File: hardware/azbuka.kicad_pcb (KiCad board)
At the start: 2 copper layers, 13 parts, among them IC1 ATTINY85-S, P1 USB_OTG, P2 CONN_01X06, Q1 MOSFET_P_CH, U1 AP111733, U2 TXS0102, U3 SJ1-3524NG

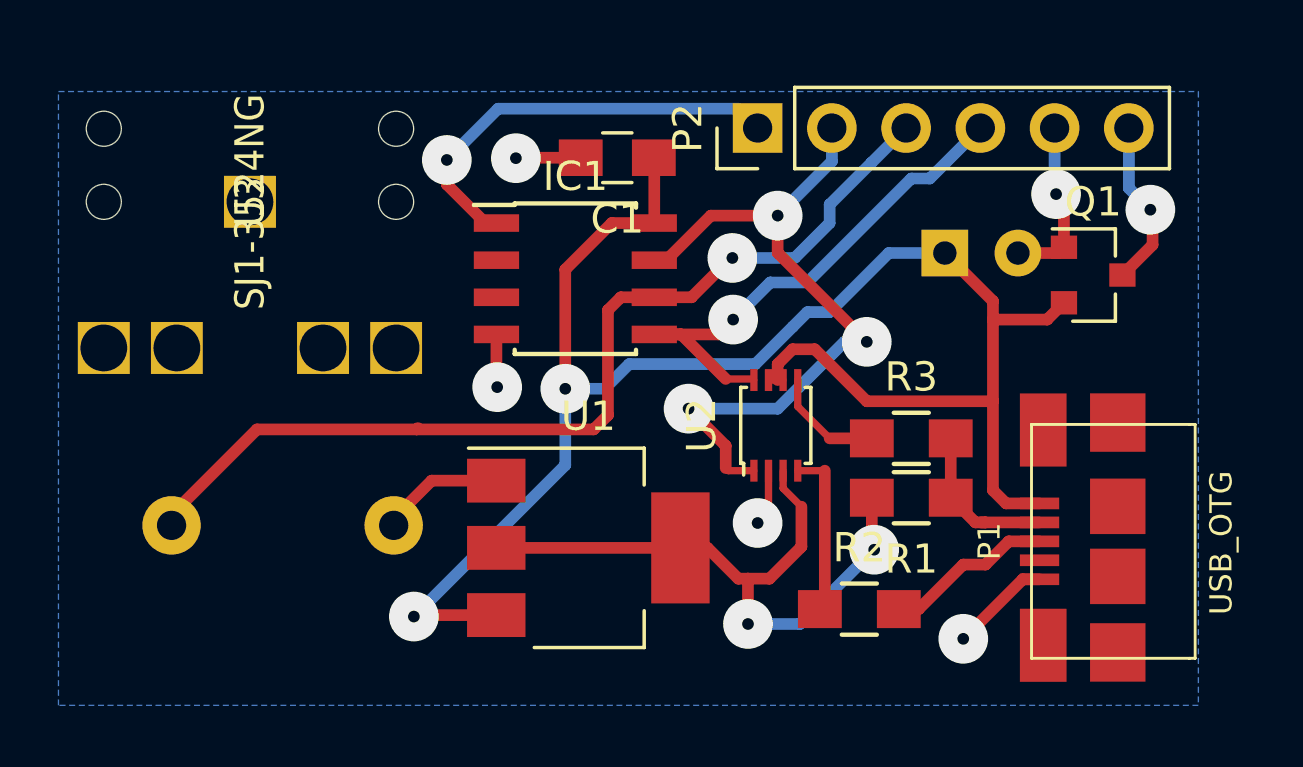
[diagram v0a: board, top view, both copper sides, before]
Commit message: Minor alterations.
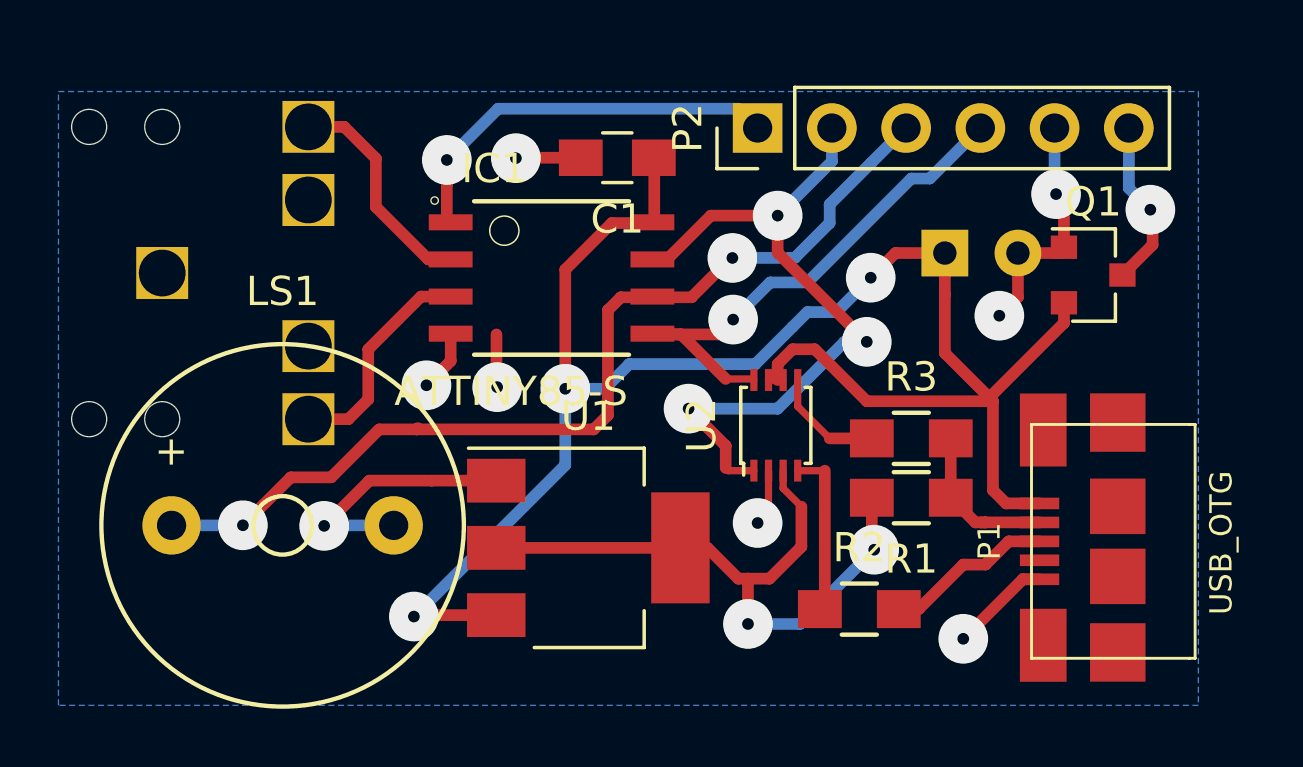
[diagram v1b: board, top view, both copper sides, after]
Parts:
- IC1: footprint azbuka:SOIC-8-1EP_3.9x4.9mm_Pitch1.27mm -> ATTINY85-20SU:SOIC127P798X216-8N
- LS1: moved to F.Cu
- U3: moved to B.Cu
- moved U3 3.87 mm to (128.6, 65.2), turned to 0 degrees
- moved IC1 0.81 mm to (141.9, 65.4)
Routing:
- net DIT: track 0.00 -> 7.72 mm
- net DAH: track 0.00 -> 7.61 mm
- net GND: track 20.2 -> 27.8 mm, vias 5 -> 7
- net (no net): track 0.00 -> 1.81 mm, vias 0 -> 1
- net +5V: track 60.4 -> 62.1 mm, vias 2 -> 3
- net RESET: track 14.7 -> 13.7 mm
- net MISO: track 33.6 -> 33.7 mm, vias 1 -> 2
